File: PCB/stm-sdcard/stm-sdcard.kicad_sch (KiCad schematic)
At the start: 3 parts, among them U1 STM32G431CBTx, U2 HX TF-CARD H1.8, U3 HX TF-CARD H1.8

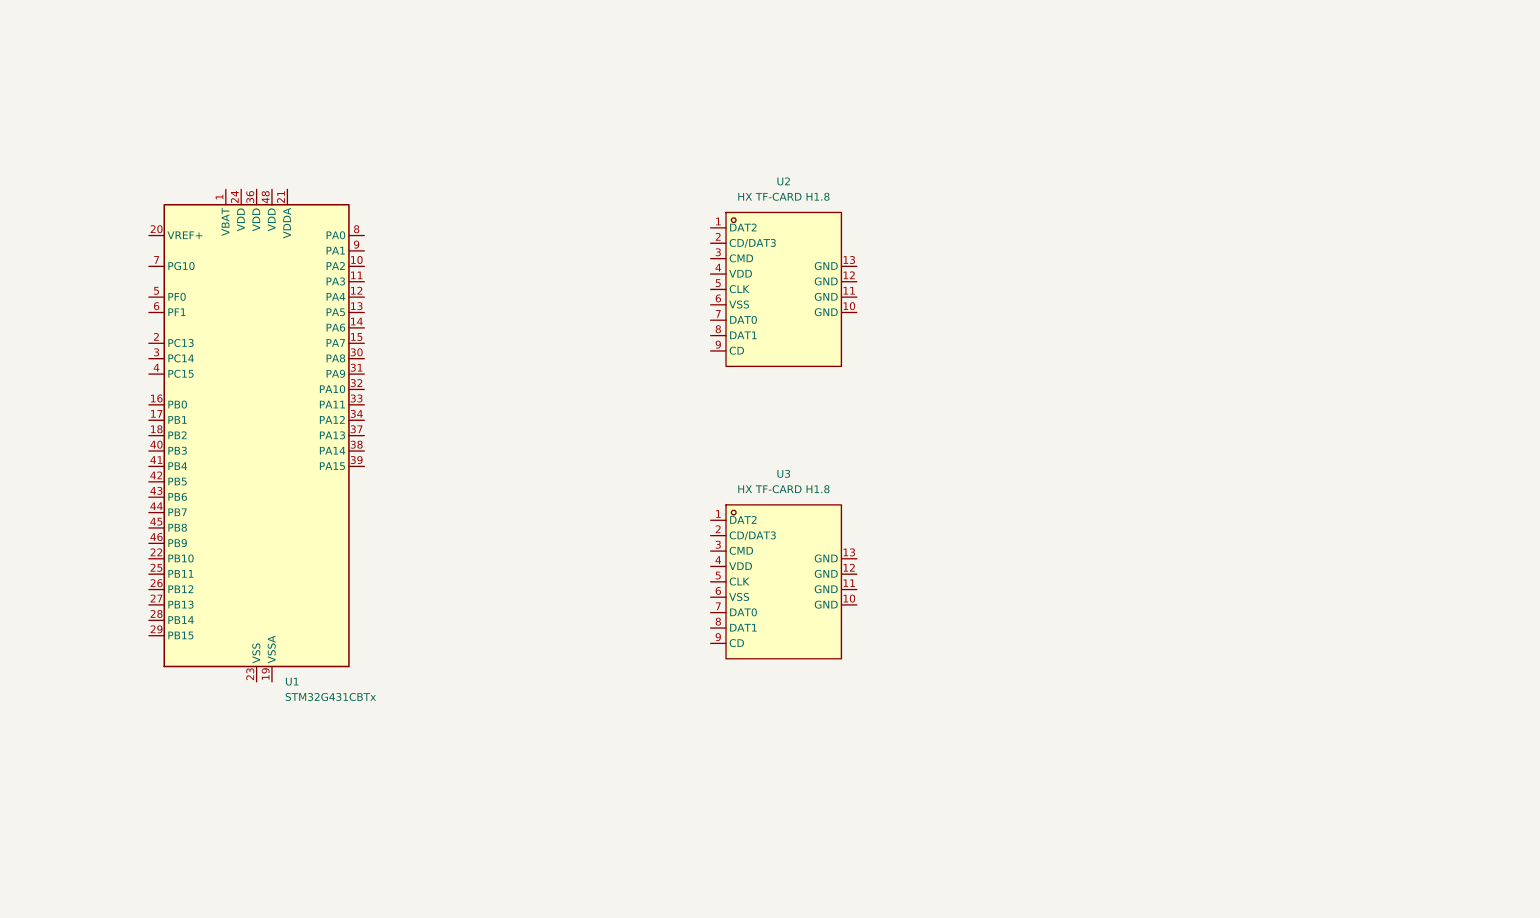
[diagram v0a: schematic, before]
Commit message: Schaltplan almost 80% finished
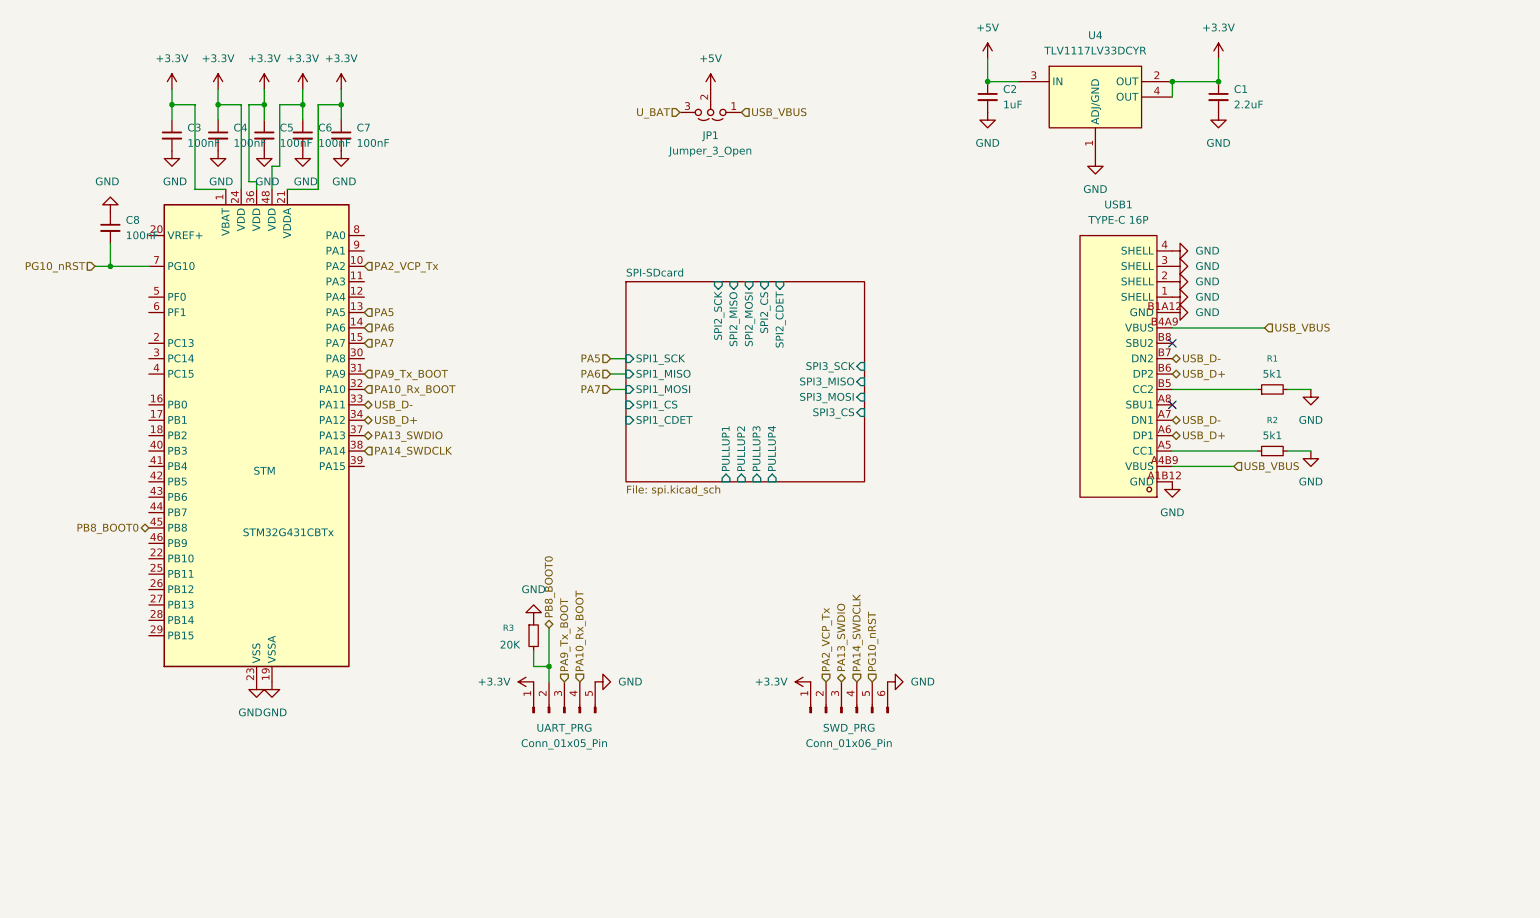
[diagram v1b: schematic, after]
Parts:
- removed U2, U3: HX TF-CARD H1.8, 1_hanxia_sd_slot:TF-SMD_HX-TF-CARD-H1.8-SY, symbol 1_hanxia_sd_slot:HXTF-CARDH1.8
- added C1: 2.2uF, symbol Device:C_Small
- added C2: 1uF, symbol Device:C_Small
- added C3, C4, C5, C6, C7, C8: 100nF, symbol Device:C_Small
- added JP1: Jumper_3_Open, symbol Jumper:Jumper_3_Open
- added R1, R2: 5k1, symbol Device:R_Small
- added R3: 20K, symbol Device:R_Small
- added SWD_PRG: Conn_01x06_Pin, symbol Connector:Conn_01x06_Pin
- added U4: TLV1117LV33DCYR, LDO-TI:SOT-223_L6.7-W3.5-P2.30-BR, symbol 3_LDO_TI:TLV1117LV33DCYR
- added UART_PRG: Conn_01x05_Pin, symbol Connector:Conn_01x05_Pin
- added USB1: TYPE-C 16P, 2_usb_C_connect:USB-C-SMD_TYPE-C16PIN_C668624, symbol 2_usb_C_connect:TYPE-C16P
- renumbered U1 to STM
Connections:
- net +3.3V: now reaches STM.1 (VBAT)
- net +3.3V: now also STM.21 (VDDA), STM.24 (VDD), STM.36 (VDD), STM.48 (VDD), C1.1, C3.1, C4.1, C5.1, C6.1, C7.1, SWD_PRG.1 (Pin_1), U4.2 (OUT), U4.4 (OUT), UART_PRG.1 (Pin_1)
- net PA2_VCP_Tx: now reaches STM.10 (PA2)
- net PA2_VCP_Tx: now also SWD_PRG.2 (Pin_2)
- net PA5: now reaches STM.13 (PA5)
- net PA6: now reaches STM.14 (PA6)
- net PA7: now reaches STM.15 (PA7)
- net GND: now reaches STM.19 (VSSA)
- net GND: now also STM.23 (VSS), STM.35 (VSS), STM.47 (VSS), C1.2, C2.2, C3.2, C4.2, C5.2, C6.2, C7.2, C8.1, R1.2, R2.2, R3.1, SWD_PRG.6 (Pin_6), U4.1 (ADJ/GND), UART_PRG.5 (Pin_5), USB1.1 (SHELL), USB1.2 (SHELL), USB1.3 (SHELL), USB1.4 (SHELL), USB1.A1B12 (GND), USB1.B1A12 (GND)
- net PA9_Tx_BOOT: now reaches STM.31 (PA9)
- net PA9_Tx_BOOT: now also UART_PRG.3 (Pin_3)
- net PA10_Rx_BOOT: now reaches STM.32 (PA10)
- net PA10_Rx_BOOT: now also UART_PRG.4 (Pin_4)
- net USB_D-: now reaches STM.33 (PA11)
- net USB_D-: now also USB1.A7 (DN1), USB1.B7 (DN2)
- net USB_D+: now reaches STM.34 (PA12)
- net USB_D+: now also USB1.A6 (DP1), USB1.B6 (DP2)
- net PA13_SWDIO: now reaches STM.37 (PA13)
- net PA13_SWDIO: now also SWD_PRG.3 (Pin_3)
- net PA14_SWDCLK: now reaches STM.38 (PA14)
- net PA14_SWDCLK: now also SWD_PRG.4 (Pin_4)
- net PB8_BOOT0: now reaches STM.45 (PB8)
- net PB8_BOOT0: now also R3.2, UART_PRG.2 (Pin_2)
- net PG10_nRST: now reaches STM.7 (PG10)
- net PG10_nRST: now also C8.2, SWD_PRG.5 (Pin_5)
- new net: R2.1, USB1.A5 (CC1)
- new net: R1.1, USB1.B5 (CC2)
- new net +5V: C2.1, JP1.2 (C), U4.3 (IN)
- new net USB_VBUS: JP1.1 (A), USB1.A4B9 (VBUS), USB1.B4A9 (VBUS)
- new net U_BAT: JP1.3 (B)
- no-connect marks 0 -> 2
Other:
- added sheet SPI-SDcard (spi.kicad_sch)

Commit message: layout almost done, error check missing, routing missing
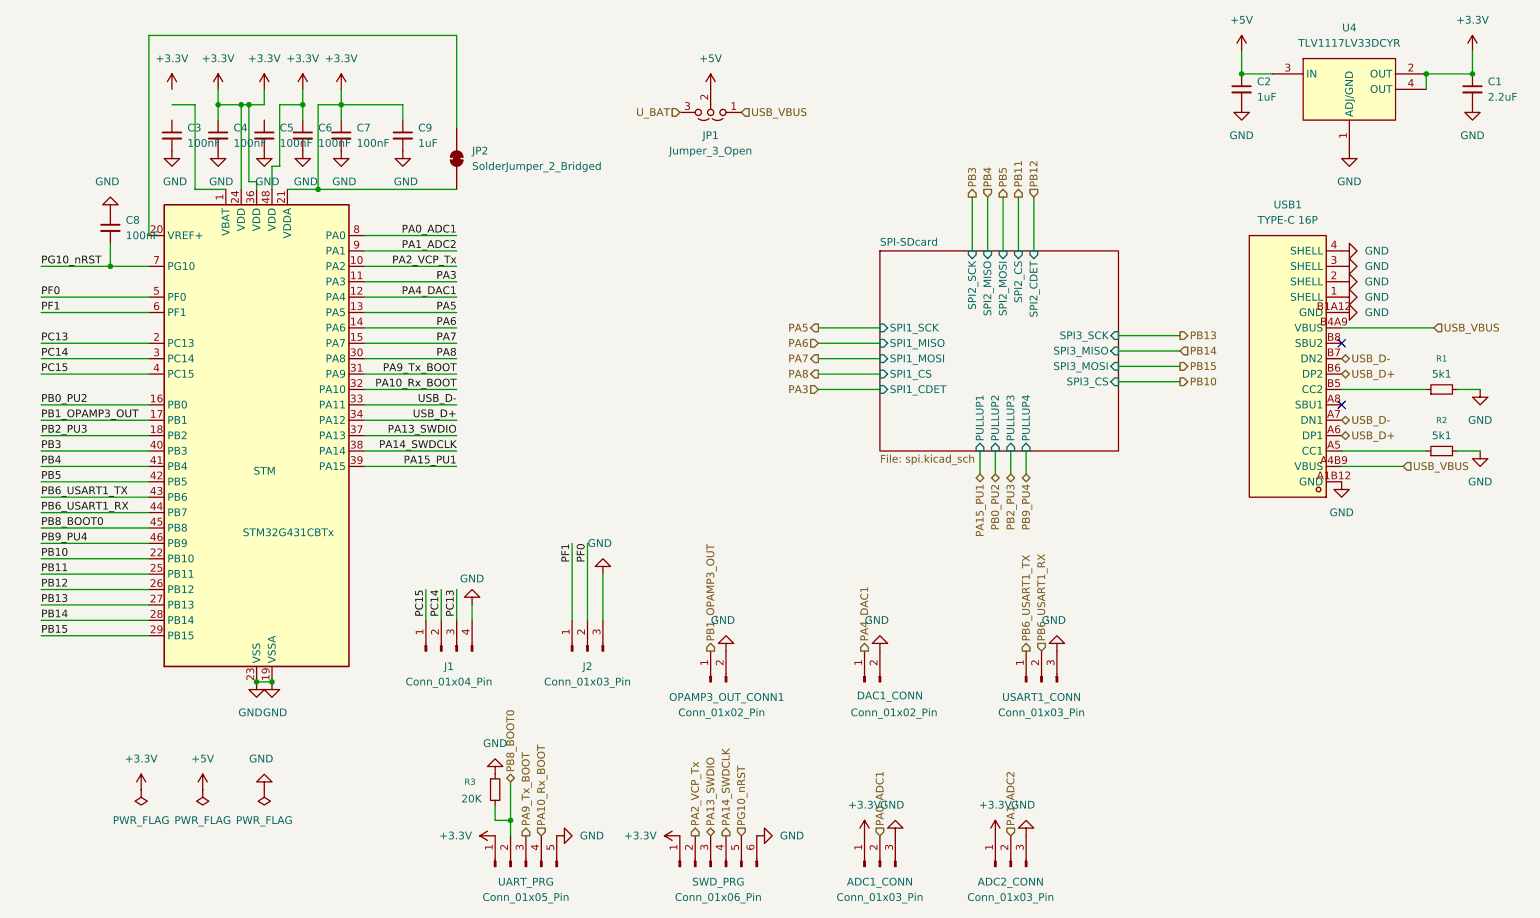
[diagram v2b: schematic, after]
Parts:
- added ADC1_CONN, ADC2_CONN, J2, USART1_CONN: Conn_01x03_Pin, symbol Connector:Conn_01x03_Pin
- added C9: 1uF, symbol Device:C_Small
- added DAC1_CONN, OPAMP3_OUT_CONN1: Conn_01x02_Pin, symbol Connector:Conn_01x02_Pin
- added J1: Conn_01x04_Pin, symbol Connector:Conn_01x04_Pin
- added JP2: SolderJumper_2_Bridged, symbol Jumper:SolderJumper_2_Bridged
- U4: footprint LDO-TI:SOT-223_L6.7-W3.5-P2.30-BR -> 3_LDO_TI:SOT-223_L6.7-W3.5-P2.30-BR
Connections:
- net +3.3V: now also ADC1_CONN.1 (Pin_1), ADC2_CONN.1 (Pin_1), C9.1, JP2.1 (A); no longer C3.1, C5.1, STM.1 (VBAT)
- net GND: now also ADC1_CONN.3 (Pin_3), ADC2_CONN.3 (Pin_3), C9.2, DAC1_CONN.2 (Pin_2), J1.4 (Pin_4), J2.3 (Pin_3), OPAMP3_OUT_CONN1.2 (Pin_2), USART1_CONN.3 (Pin_3)
- net PA3: now reaches STM.11 (PA3)
- net PA4_DAC1: now reaches STM.12 (PA4)
- net PA4_DAC1: now also DAC1_CONN.1 (Pin_1)
- net PB0_PU2: now reaches STM.16 (PB0)
- net PB1_OPAMP3_OUT: now reaches STM.17 (PB1)
- net PB1_OPAMP3_OUT: now also OPAMP3_OUT_CONN1.1 (Pin_1)
- net PB2_PU3: now reaches STM.18 (PB2)
- net PC13: now reaches STM.2 (PC13)
- net PC13: now also J1.3 (Pin_3)
- net at STM.20 (VREF+): now also JP2.2 (B)
- net PB10: now reaches STM.22 (PB10)
- net PB11: now reaches STM.25 (PB11)
- net PB12: now reaches STM.26 (PB12)
- net PB13: now reaches STM.27 (PB13)
- net PB14: now reaches STM.28 (PB14)
- net PB15: now reaches STM.29 (PB15)
- net PC14: now reaches STM.3 (PC14)
- net PC14: now also J1.2 (Pin_2)
- net PA8: now reaches STM.30 (PA8)
- net PA15_PU1: now reaches STM.39 (PA15)
- net PC15: now reaches STM.4 (PC15)
- net PC15: now also J1.1 (Pin_1)
- net PB3: now reaches STM.40 (PB3)
- net PB4: now reaches STM.41 (PB4)
- net PB5: now reaches STM.42 (PB5)
- net PB6_USART1_TX: now reaches STM.43 (PB6)
- net PB6_USART1_TX: now also USART1_CONN.1 (Pin_1)
- net PB6_USART1_RX: now reaches STM.44 (PB7)
- net PB6_USART1_RX: now also USART1_CONN.2 (Pin_2)
- net PB9_PU4: now reaches STM.46 (PB9)
- net PF0: now reaches STM.5 (PF0)
- net PF0: now also J2.2 (Pin_2)
- net PF1: now reaches STM.6 (PF1)
- net PF1: now also J2.1 (Pin_1)
- net PA0_ADC1: now reaches STM.8 (PA0)
- net PA0_ADC1: now also ADC1_CONN.2 (Pin_2)
- net PA1_ADC2: now reaches STM.9 (PA1)
- net PA1_ADC2: now also ADC2_CONN.2 (Pin_2)
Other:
- moved on the sheet: C1, C2, R1, R2, R3, SWD_PRG, U4, UART_PRG, USB1
